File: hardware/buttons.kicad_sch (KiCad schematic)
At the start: 9 parts, among them SW1 SW_Push_Open, SW2 SW_Push_Open, SW3 SW_Push_Open

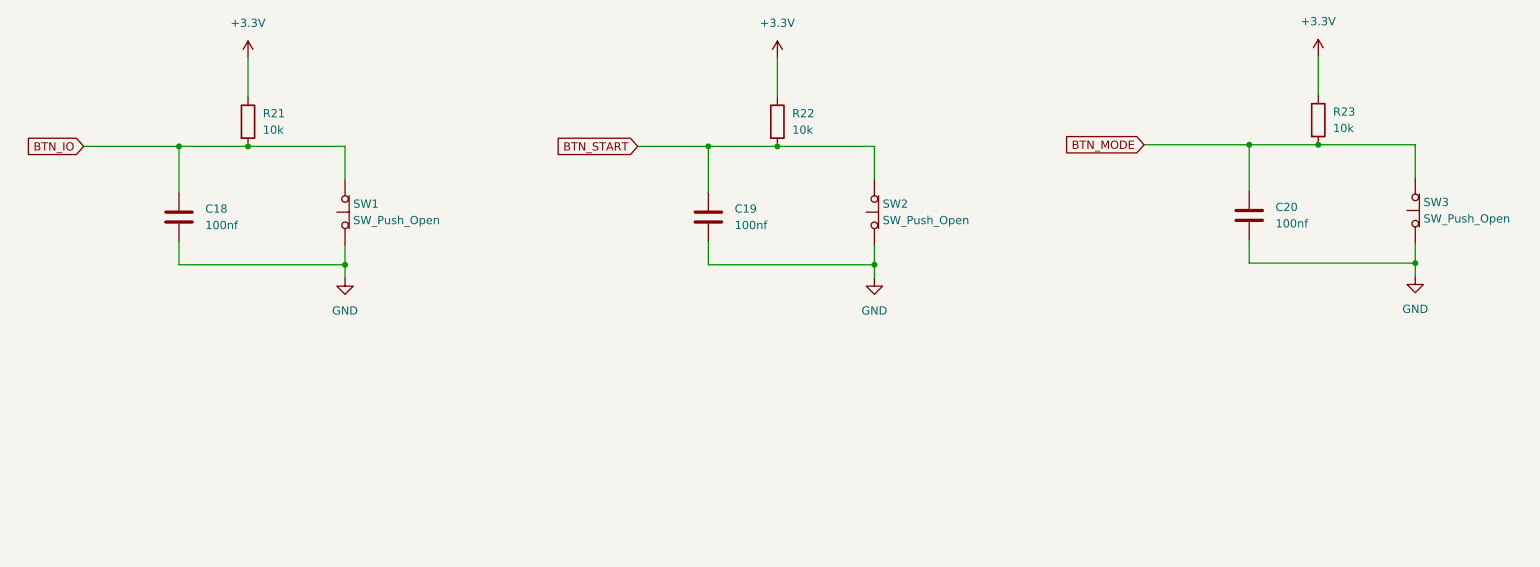
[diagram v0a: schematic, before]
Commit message: Flow module completed
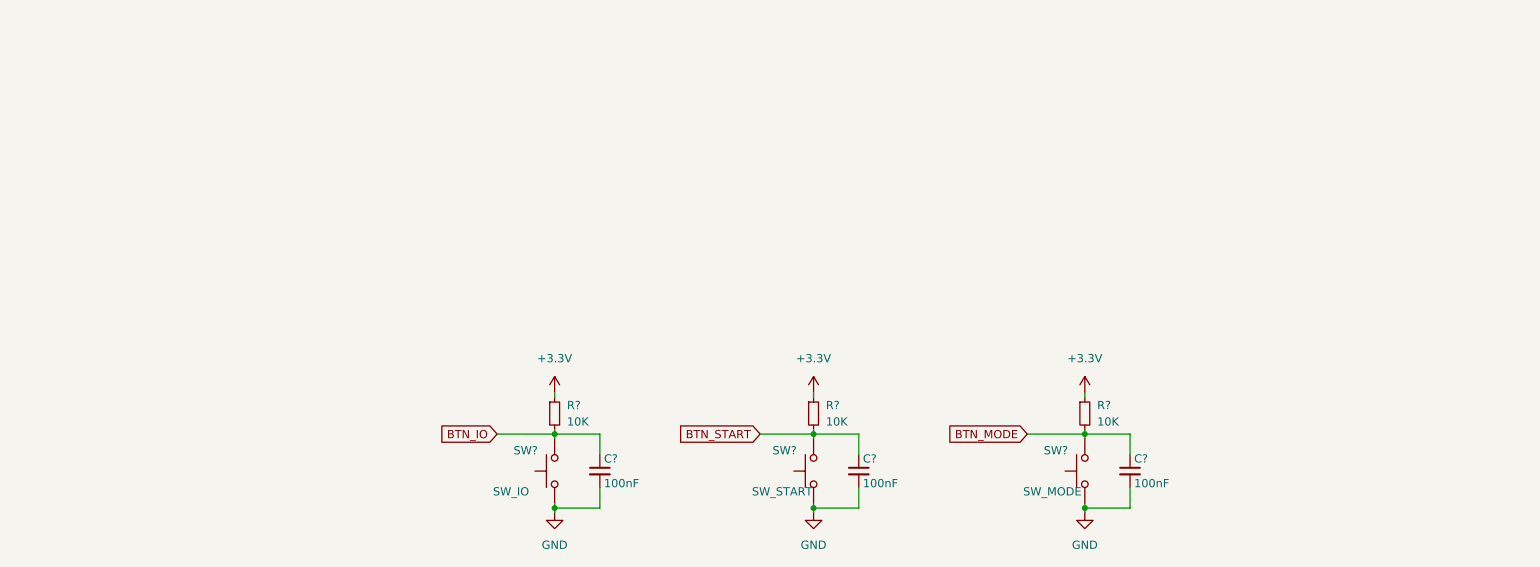
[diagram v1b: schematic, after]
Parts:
- removed C18, C19, C20: 100nf, symbol Device:C
- removed R21, R22, R23: 10k, symbol Device:R
- removed SW1, SW2, SW3: SW_Push_Open, symbol Switch:SW_Push_Open
- added C? (x3): 100nF, symbol Device:C_Small
- added R? (x3): 10K, symbol Device:R_Small
- added SW?: SW_START, symbol Switch:SW_Push
- added SW?: SW_MODE, symbol Switch:SW_Push
- added SW?: SW_IO, symbol Switch:SW_Push
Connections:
- net +3.3V: now also R?.1, R?.1, R?.1
- net BTN_IO: now also C?.1, R?.2, SW?.2
- net BTN_MODE: now also C?.1, R?.2, SW?.2
- net BTN_START: now also C?.1, R?.2, SW?.2
- net GND: now also C?.2, C?.2, C?.2, SW?.1, SW?.1, SW?.1
